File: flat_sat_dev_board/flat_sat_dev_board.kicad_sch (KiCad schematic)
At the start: 0 parts

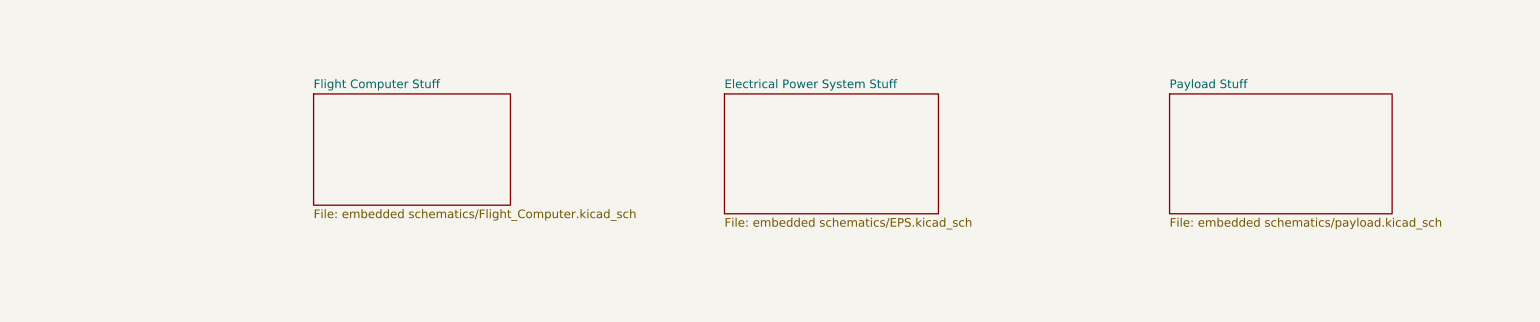
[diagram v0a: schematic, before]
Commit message: Updated all the Diodes!
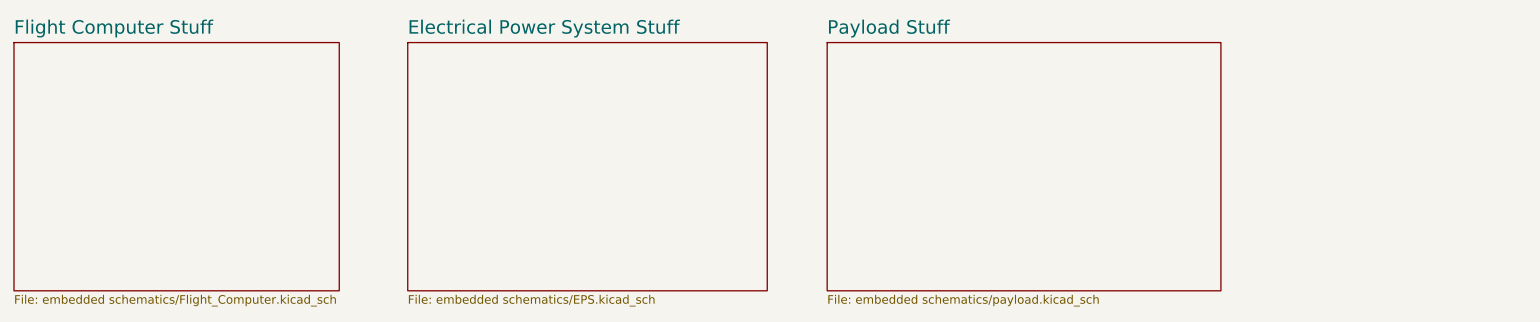
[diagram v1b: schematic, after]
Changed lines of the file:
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@@
 	)
 	(sheet
-		(at 82.55 90.17)
-		(size 29.21 16.51)
+		(at 38.1 82.55)
+		(size 48.26 36.83)
 		(fields_autoplaced yes)
 		(stroke
@@
 		)
 		(property "Sheetname" "Flight Computer Stuff"
-			(at 82.55 89.4584 0)
+			(at 38.1 81.4734 0)
 			(effects
 				(font
-					(size 1.27 1.27)
+					(size 2 2)
 				)
 				(justify left bottom)
@@
 		)
 		(property "Sheetfile" "embedded schematics/Flight_Computer.kicad_sch"
-			(at 82.55 107.2646 0)
+			(at 38.1 119.9646 0)
 			(effects
 				(font
@@
 	)
 	(sheet
-		(at 209.55 90.17)
-		(size 33.02 17.78)
+		(at 158.75 82.55)
+		(size 58.42 36.83)
 		(fields_autoplaced yes)
 		(stroke
@@
 		)
 		(property "Sheetname" "Payload Stuff"
-			(at 209.55 89.4584 0)
+			(at 158.75 81.4734 0)
 			(effects
 				(font
-					(size 1.27 1.27)
+					(size 2 2)
 				)
 				(justify left bottom)
@@
 		)
 		(property "Sheetfile" "embedded schematics/payload.kicad_sch"
-			(at 209.55 108.5346 0)
+			(at 158.75 119.9646 0)
 			(effects
 				(font
@@
 	)
 	(sheet
-		(at 143.51 90.17)
-		(size 31.75 17.78)
+		(at 96.52 82.55)
+		(size 53.34 36.83)
 		(fields_autoplaced yes)
 		(stroke
@@
 		)
 		(property "Sheetname" "Electrical Power System Stuff"
-			(at 143.51 89.4584 0)
+			(at 96.52 81.4734 0)
 			(effects
 				(font
-					(size 1.27 1.27)
+					(size 2 2)
 				)
 				(justify left bottom)
@@
 		)
 		(property "Sheetfile" "embedded schematics/EPS.kicad_sch"
-			(at 143.51 108.5346 0)
+			(at 96.52 119.9646 0)
 			(effects
 				(font
